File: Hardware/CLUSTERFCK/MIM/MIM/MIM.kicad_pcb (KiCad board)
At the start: 2 copper layers, 142.1 x 108 mm, 26 parts, among them J1 Conn_02x20_Counter_Clockwise, J2 Conn_02x20_Counter_Clockwise, U1 74LS00, U10 74LS245, U2 INTEL2716, U3 INTEL2716, U4 74LS161, U5 INTEL2716, U6 74LS245, U7 74LS245, U8 74LS245, U9 74LS245

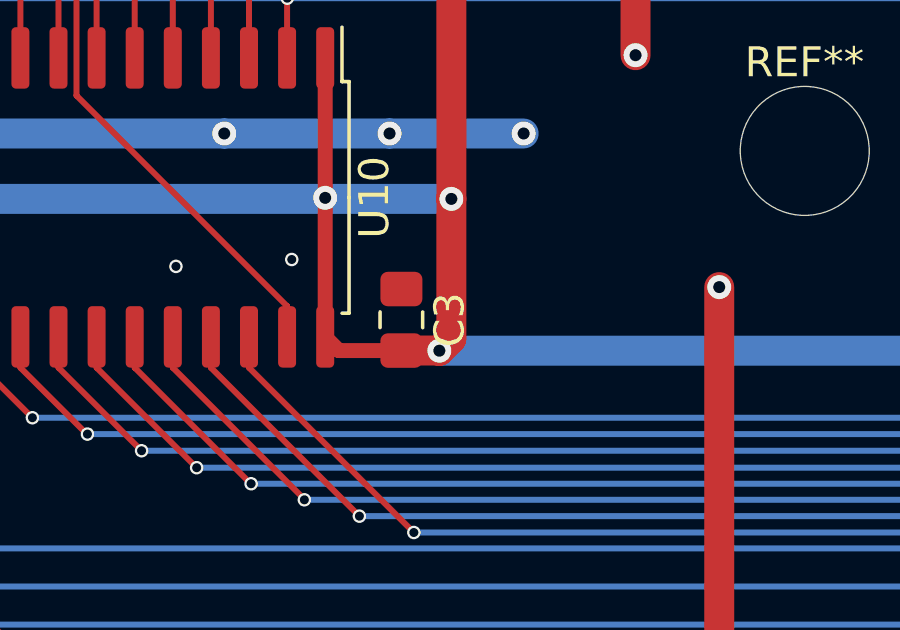
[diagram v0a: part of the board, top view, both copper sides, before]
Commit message: 0072 | 3h | make silkscreen prettier
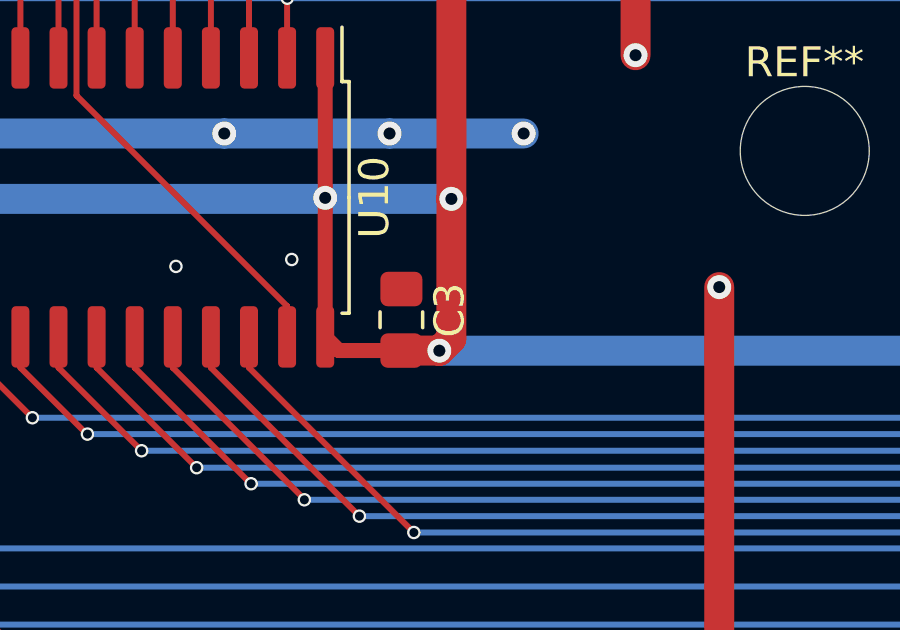
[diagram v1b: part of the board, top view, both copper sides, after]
